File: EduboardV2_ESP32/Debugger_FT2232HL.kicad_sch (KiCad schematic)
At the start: 52 parts, among them Q1 S8050_C139514, Q2 S8050_C139514, U2 FT2232HL, U3 M93C46-WMN6TP, Y1 12MHz

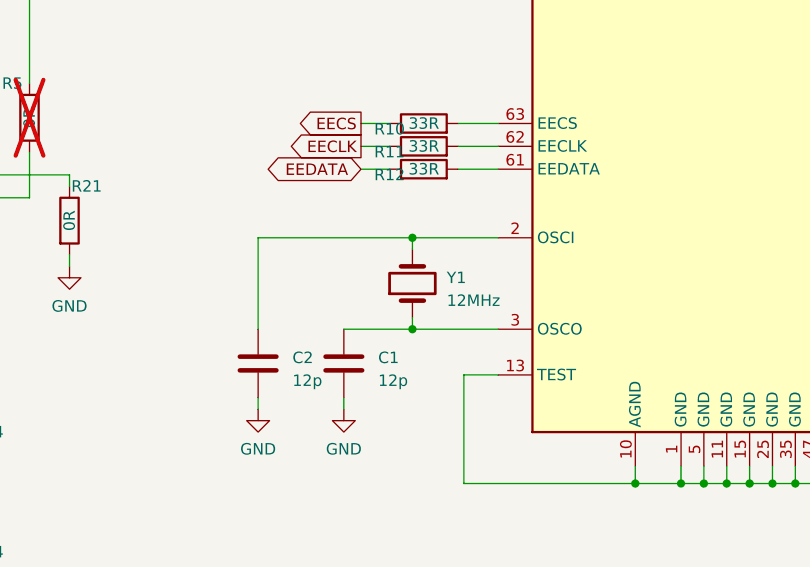
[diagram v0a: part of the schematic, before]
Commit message: all parts placed. descision about usb-debug line to be made...
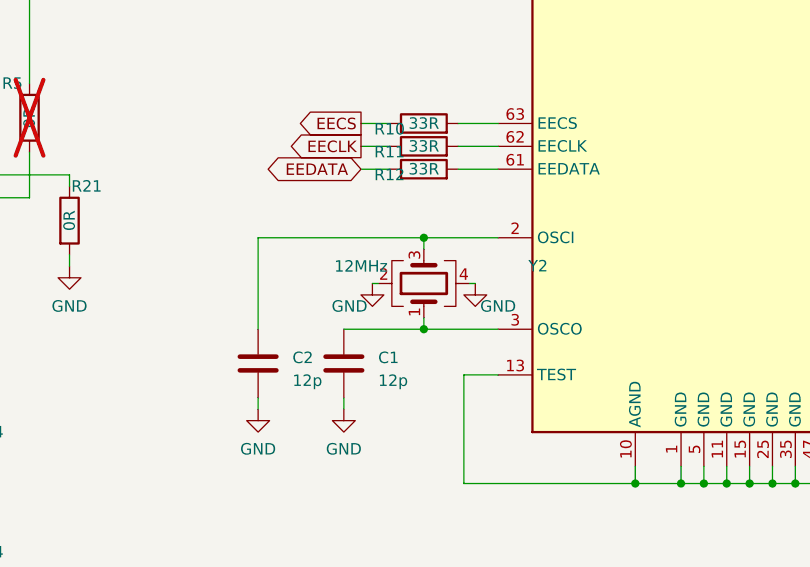
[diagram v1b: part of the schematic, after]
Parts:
- removed Y1: 12MHz, symbol Device:Crystal
- added Y2: 12MHz, Crystal:Crystal_SMD_3225-4Pin_3.2x2.5mm, symbol Device:Crystal_GND24
- C1, C10, C11, C12, C13, C14, C15, C16, C2, C3, C8, C9: footprint (none) -> Capacitor_SMD:C_0603_1608Metric
- C4, C5, C6, C7: footprint (none) -> Capacitor_SMD:C_0805_2012Metric
- D1, D2, D3: JLCPCB Part # (none) -> C383211
- FB1, FB2: footprint (none) -> Inductor_SMD:L_0805_2012Metric; JLCPCB Part # (none) -> C44838
- LED1, LED2: JLCPCB Part # (none) -> C72041
- Q1, Q2: JLCPCB Part # (none) -> C139514
- R1, R10, R11, R12, R13, R14, R15, R16, R17, R18, R2, R21, R3, R4, R5, R6, R7, R8, R9: footprint (none) -> Resistor_SMD:R_0603_1608Metric
- U2: LCSC Part (none) -> C27882
- U3: footprint SOIC-8_L4.9-W3.9-P1.27-LS6.0-BL -> JLCPCB:SOIC-8_L4.9-W3.9-P1.27-LS6.0-BL; JLCPCB Part # (none) -> C7565
- USBC1: JLCPCB Part # (none) -> C167321
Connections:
- net GND: now also Y2.2, Y2.4
- net at C2.1, U2.2 (OSCI): now also Y2.3
- net at C1.1, U2.3 (OSCO): now also Y2.1
